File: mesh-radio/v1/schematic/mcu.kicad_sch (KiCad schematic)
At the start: 34 parts, among them U9 NRF52840-QIAA-F-R7, Y1 32MHz, Y2 32.768kHz

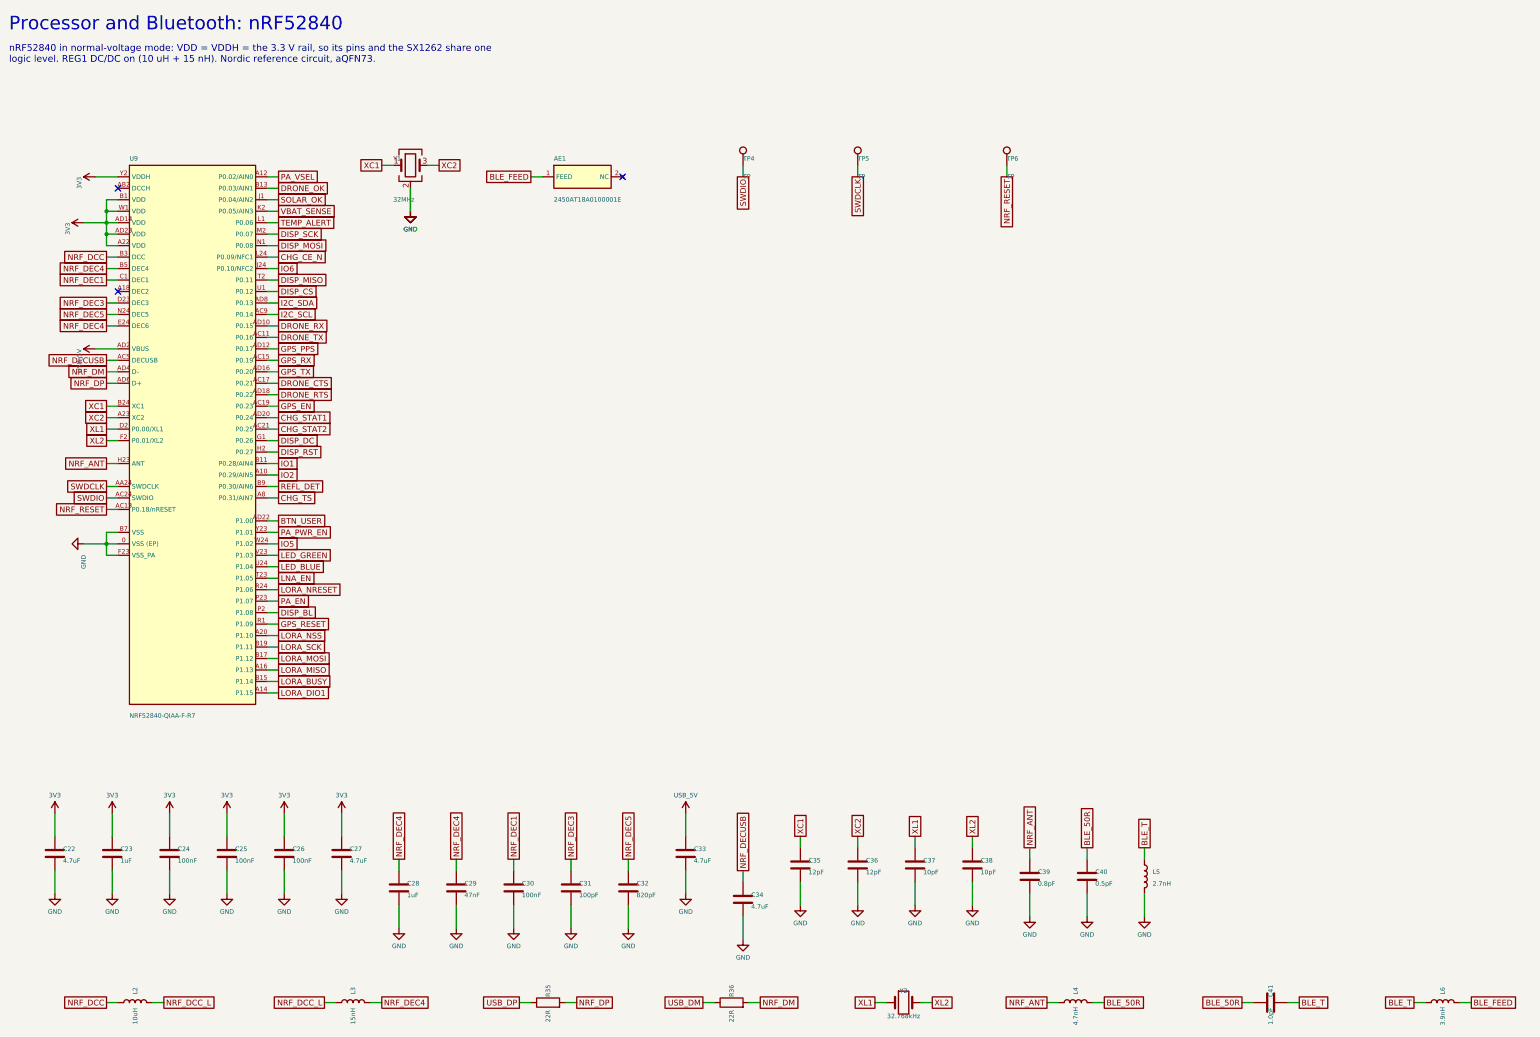
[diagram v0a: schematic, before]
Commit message: Mesh radio v1: power-path and firmware rework in progress (snapshot)
Co-Authored-By: Claude Opus 5.5 <noreply@anthropic.com>
Claude-Session: https://claude.ai/code/session_015TBB2ThqxHSgA8MkFosmn9
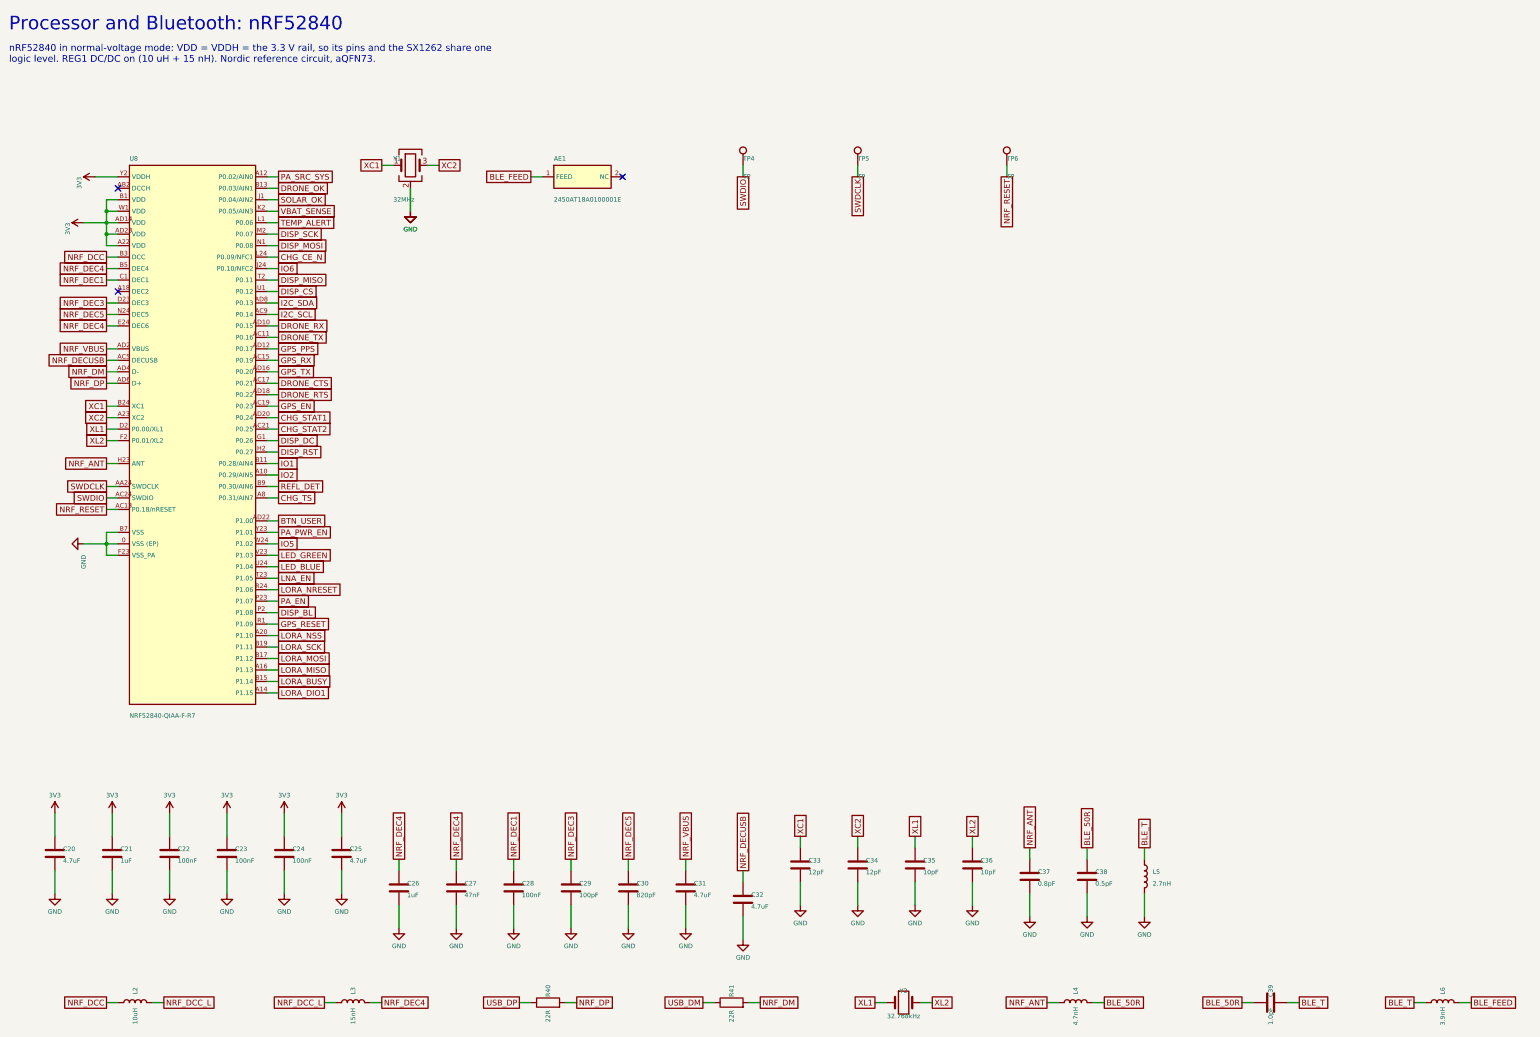
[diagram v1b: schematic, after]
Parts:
- removed C40: 0.5pF, og:C_0402, symbol Device:C
- removed C41: 1.0pF, og:C_0402, symbol Device:C
- removed R35, R36: 22R, og:R_0402, symbol Device:R
- removed U9: NRF52840-QIAA-F-R7, og:AQFN-73_L7.0-W7.0-P0.50-BL-EP4.8, symbol og:NRF52840
- added C20: 4.7uF, og:C_0603, symbol Device:C
- added C21: 1uF, og:C_0402, symbol Device:C
- added R40, R41: 22R, og:R_0402, symbol Device:R
- added U8: NRF52840-QIAA-F-R7, og:AQFN-73_L7.0-W7.0-P0.50-BL-EP4.8, symbol og:NRF52840
- C22: value 4.7uF -> 100nF; footprint og:C_0603 -> og:C_0402; DigiKey 1276-1044-1-ND -> 1276-1001-1-ND; LCSC C1705 -> C1525; MPN CL10A475KP8NNNC -> CL05B104KO5NNNC
- C23, C28: value 1uF -> 100nF; DigiKey 1276-1067-1-ND -> 1276-1001-1-ND; LCSC C29266 -> C1525; MPN CL05A105KO5NNNC -> CL05B104KO5NNNC
- C25: value 100nF -> 4.7uF; footprint og:C_0402 -> og:C_0603; DigiKey 1276-1001-1-ND -> 1276-1044-1-ND; LCSC C1525 -> C1705; MPN CL05B104KO5NNNC -> CL10A475KP8NNNC
- C26: value 100nF -> 1uF; DigiKey 1276-1001-1-ND -> 1276-1067-1-ND; LCSC C1525 -> C29266; MPN CL05B104KO5NNNC -> CL05A105KO5NNNC
- C27: value 4.7uF -> 47nF; footprint og:C_0603 -> og:C_0402; DigiKey 1276-1044-1-ND -> 1276-1077-1-ND; LCSC C1705 -> C307434; MPN CL10A475KP8NNNC -> CL05B473KO5NNNC
- C29: value 47nF -> 100pF; DigiKey 1276-1077-1-ND -> 490-5922-1-ND; LCSC C307434 -> C77177; MPN CL05B473KO5NNNC -> GRM1555C1H101JA01D; Manufacturer Samsung Electro-Mechanics -> Murata
- C30: value 100nF -> 820pF; DigiKey 1276-1001-1-ND -> 490-3242-1-ND; LCSC C1525 -> C85943; MPN CL05B104KO5NNNC -> GRM1555C1H821JA01D; Manufacturer Samsung Electro-Mechanics -> Murata
- C31: value 100pF -> 4.7uF; footprint og:C_0402 -> og:C_0603; DigiKey 490-5922-1-ND -> 1276-1044-1-ND; LCSC C77177 -> C1705; MPN GRM1555C1H101JA01D -> CL10A475KP8NNNC; Manufacturer Murata -> Samsung Electro-Mechanics
- C32: value 820pF -> 4.7uF; footprint og:C_0402 -> og:C_0603; DigiKey 490-3242-1-ND -> 1276-1044-1-ND; LCSC C85943 -> C1705; MPN GRM1555C1H821JA01D -> CL10A475KP8NNNC; Manufacturer Murata -> Samsung Electro-Mechanics
- C33, C34: value 4.7uF -> 12pF; footprint og:C_0603 -> og:C_0402; DigiKey 1276-1044-1-ND -> 1276-1178-1-ND; LCSC C1705 -> C26406; MPN CL10A475KP8NNNC -> CL05C120JB5NNNC
- C35, C36: value 12pF -> 10pF; DigiKey 1276-1178-1-ND -> 490-3113-1-ND; LCSC C26406 -> C85874; MPN CL05C120JB5NNNC -> GJM1555C1H100JB01D; Manufacturer Samsung Electro-Mechanics -> Murata
- C37: value 10pF -> 0.8pF; DigiKey 490-3113-1-ND -> 490-11253-1-ND; LCSC C85874 -> C88902; MPN GJM1555C1H100JB01D -> GJM1555C1HR80WB01D
- C38: value 10pF -> 0.5pF; DigiKey 490-3113-1-ND -> 490-6077-1-ND; LCSC C85874 -> C76911; MPN GJM1555C1H100JB01D -> GJM1555C1HR50BB01D
- C39: value 0.8pF -> 1.0pF; DigiKey 490-11253-1-ND -> 490-6073-1-ND; LCSC C88902 -> C76898; MPN GJM1555C1HR80WB01D -> GJM1555C1H1R0BB01D
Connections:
- net USB_5V is gone; now on net XC1: C33.1
- net 3V3: now also C20.1, C21.1, U8.A22 (VDD), U8.AD14 (VDD), U8.AD23 (VDD), U8.B1 (VDD), U8.W1 (VDD), U8.Y2 (VDDH); no longer C26.1, C27.1
- net BLE_50R: now also C38.1, C39.1
- net BLE_T: now also C39.2
- net BTN_USER: now also U8.AD22 (P1.00)
- net CHG_CE_N: now also U8.L24 (P0.09/NFC1)
- net CHG_STAT1: now also U8.AD20 (P0.24)
- net CHG_STAT2: now also U8.AC21 (P0.25)
- net CHG_TS: now also U8.A8 (P0.31/AIN7)
- net DISP_BL: now also U8.P2 (P1.08)
- net DISP_CS: now also U8.U1 (P0.12)
- net DISP_DC: now also U8.G1 (P0.26)
- net DISP_MISO: now also U8.T2 (P0.11)
- net DISP_MOSI: now also U8.N1 (P0.08)
- net DISP_RST: now also U8.H2 (P0.27)
- net DISP_SCK: now also U8.M2 (P0.07)
- net DRONE_CTS: now also U8.AC17 (P0.21)
- net DRONE_OK: now also U8.B13 (P0.03/AIN1)
- net DRONE_RTS: now also U8.AD18 (P0.22)
- net DRONE_RX: now also U8.AD10 (P0.15)
- net DRONE_TX: now also U8.AC11 (P0.16)
- net GND: now also C20.2, C21.2, U8.0 (VSS (EP)), U8.B7 (VSS), U8.F23 (VSS_PA); no longer C39.2
- net GPS_EN: now also U8.AC19 (P0.23)
- net GPS_PPS: now also U8.AD12 (P0.17)
- net GPS_RESET: now also U8.R1 (P1.09)
- net GPS_RX: now also U8.AC15 (P0.19)
- net GPS_TX: now also U8.AD16 (P0.20)
- net I2C_SCL: now also U8.AC9 (P0.14)
- net I2C_SDA: now also U8.AD8 (P0.13)
- net IO1: now also U8.B11 (P0.28/AIN4)
- net IO2: now also U8.A10 (P0.29/AIN5)
- net IO5: now also U8.W24 (P1.02)
- net IO6: now also U8.J24 (P0.10/NFC2)
- net LED_BLUE: now also U8.U24 (P1.04)
- net LED_GREEN: now also U8.V23 (P1.03)
- net LNA_EN: now also U8.T23 (P1.05)
- net LORA_BUSY: now also U8.B15 (P1.14)
- net LORA_DIO1: now also U8.A14 (P1.15)
- net LORA_MISO: now also U8.A16 (P1.13)
- net LORA_MOSI: now also U8.B17 (P1.12)
- net LORA_NRESET: now also U8.R24 (P1.06)
- net LORA_NSS: now also U8.A20 (P1.10)
- net LORA_SCK: now also U8.B19 (P1.11)
- net NRF_ANT: now also C37.1, U8.H23 (ANT); no longer C39.1
- net NRF_DCC: now also U8.B3 (DCC)
- net NRF_DEC1: now also C28.1, U8.C1 (DEC1); no longer C30.1
- net NRF_DEC3: now also C29.1, U8.D23 (DEC3); no longer C31.1
- net NRF_DEC4: now also C26.1, C27.1, U8.B5 (DEC4), U8.E24 (DEC6); no longer C28.1, C29.1
- net NRF_DEC5: now also C30.1, U8.N24 (DEC5); no longer C32.1
- net NRF_DECUSB: now also C32.1, U8.AC5 (DECUSB); no longer C34.1
- net NRF_DM: now also R41.2, U8.AD4 (D-)
- net NRF_DP: now also R40.2, U8.AD6 (D+)
- net NRF_RESET: now also U8.AC13 (P0.18/nRESET)
- net PA_EN: now also U8.P23 (P1.07)
- net PA_PWR_EN: now also U8.Y23 (P1.01)
- net REFL_DET: now also U8.B9 (P0.30/AIN6)
- net SOLAR_OK: now also U8.J1 (P0.04/AIN2)
- net SWDCLK: now also U8.AA24 (SWDCLK)
- net SWDIO: now also U8.AC24 (SWDIO)
- net TEMP_ALERT: now also U8.L1 (P0.06)
- net USB_DM: now also R41.1
- net USB_DP: now also R40.1
- net VBAT_SENSE: now also U8.K2 (P0.05/AIN3)
- net XC1: now also U8.B24 (XC1); no longer C35.1
- net XC2: now also C34.1, U8.A23 (XC2); no longer C36.1
- net XL1: now also C35.1, U8.D2 (P0.00/XL1); no longer C37.1
- net XL2: now also C36.1, U8.F2 (P0.01/XL2); no longer C38.1
- new net NRF_VBUS: C31.1, U8.AD2 (VBUS)
- new net PA_SRC_SYS: U8.A12 (P0.02/AIN0)
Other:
- moved on the sheet: C22, C23, C24, C25, C26, C27, C28, C29, C30, C31, C32, C33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
